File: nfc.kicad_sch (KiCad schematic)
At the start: 16 parts, among them Y1 Crystal_GND24

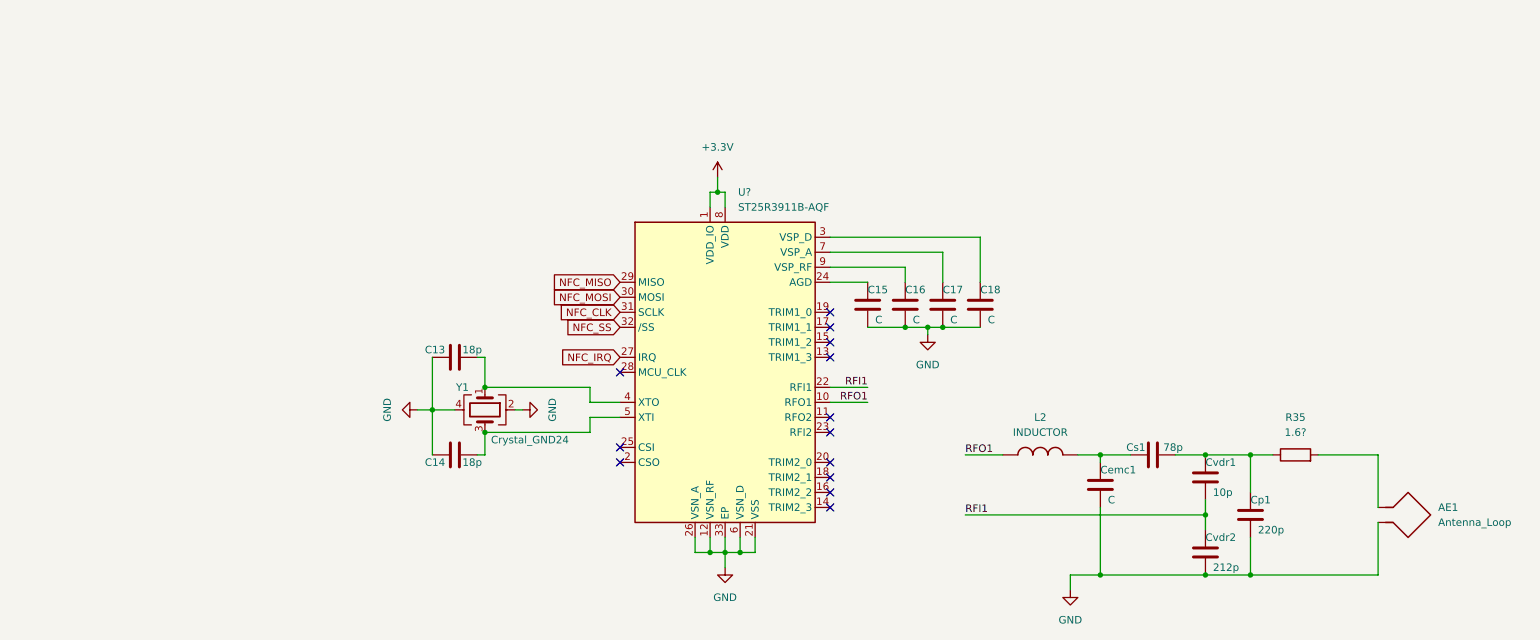
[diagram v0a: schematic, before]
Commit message: Almost finalize schematics
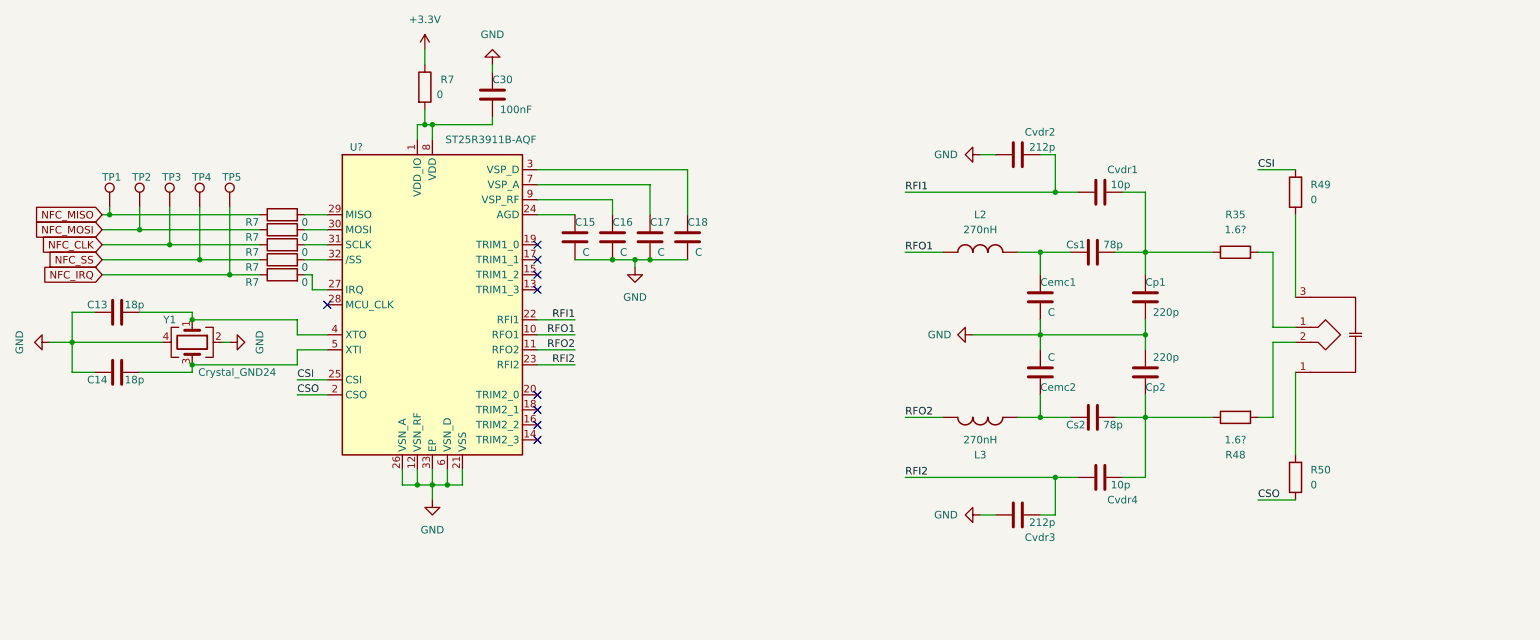
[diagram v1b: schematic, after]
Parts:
- removed AE1: Antenna_Loop, symbol Device:Antenna_Loop
- added C30: 100nF, Capacitor_SMD:C_0603_1608Metric, symbol Device:C
- added Cemc2: C, Capacitor_SMD:C_0603_1608Metric, symbol Device:C
- added Cp2: 220p, Capacitor_SMD:C_0603_1608Metric, symbol Device:C
- added Cs2: 78p, Capacitor_SMD:C_0603_1608Metric, symbol Device:C
- added Cvdr3: 212p, Capacitor_SMD:C_0603_1608Metric, symbol Device:C
- added Cvdr4: 10p, Capacitor_SMD:C_0603_1608Metric, symbol Device:C
- added L3: 270nH, Inductor_SMD:L_1210_3225Metric, symbol _GRZ_Passive:INDUCTOR
- added R48: 1.6?, _Resistors_GRZ:R_0603, symbol Device:R
- added R49, R50: 0, _Resistors_GRZ:R_0603, symbol Device:R
- added R7 (x6): 0, Resistor_SMD:R_0603_1608Metric, symbol Device:R
- added TP1, TP2, TP3, TP4, TP5: TestPoint, TestPoint:TestPoint_Pad_D2.0mm, symbol Connector:TestPoint
- added U7: ~, myFootprints:NFC_antenna, symbol mySymbols:NFC_antenna
- L2: value INDUCTOR -> 270nH; footprint (none) -> Inductor_SMD:L_1210_3225Metric
- R35: footprint (none) -> _Resistors_GRZ:R_0603
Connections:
- net +3.3V: now also R7.1; no longer U?.1 (VDD_IO), U?.8 (VDD)
- net GND: now also Cvdr2.2, C30.2, Cemc2.1, Cp2.1, Cvdr3.2; no longer Cvdr2.1
- net NFC_CLK: now also R7.1, TP3.1; no longer U?.31 (SCLK)
- net NFC_IRQ: now also R7.1, TP5.1; no longer U?.27 (IRQ)
- net NFC_MISO: now also R7.1, TP1.1; no longer U?.29 (MISO)
- net NFC_MOSI: now also R7.1, TP2.1; no longer U?.30 (MOSI)
- net NFC_SS: now also R7.1, TP4.1; no longer U?.32 (/SS)
- net RFI1: now also Cvdr1.2, Cvdr2.1; no longer Cvdr1.1, Cvdr2.2
- net at Cp1.2, Cs1.1, R35.1: now also Cvdr1.1; no longer Cvdr1.2
- net RFO2: now reaches U?.11 (RFO2)
- net RFO2: now also L3.1
- net CSO: now reaches U?.2 (CSO)
- net CSO: now also R50.1
- net RFI2: now reaches U?.23 (RFI2)
- net RFI2: now also Cvdr3.1, Cvdr4.2
- net CSI: now reaches U?.25 (CSI)
- net CSI: now also R49.2
- net at R35.2: now also U7.1
- new net: R7.2, U?.30 (MOSI)
- new net: R49.1, U7.3
- new net: C30.1, R7.2, U?.1 (VDD_IO), U?.8 (VDD)
- new net: R7.2, U?.27 (IRQ)
- new net: R7.2, U?.29 (MISO)
- new net: R7.2, U?.31 (SCLK)
- new net: R7.2, U?.32 (/SS)
- new net: Cp2.2, Cs2.1, Cvdr4.1, R48.1
- new net: Cemc2.2, Cs2.2, L3.2
- new net: R50.2, U7.1
- new net: R48.2, U7.2
- no-connect marks 13 -> 9
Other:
- moved on the sheet: C13, C14, C15, C16, C17, C18, Cemc1, Cp1, Cs1, Cvdr1, Cvdr2, L2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
